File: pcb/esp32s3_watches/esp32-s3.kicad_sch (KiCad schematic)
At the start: 14 parts, among them J2 10067847-001RLF, U1 ESP32-S3-DevKitC, U4 SW_DPDT_XLX

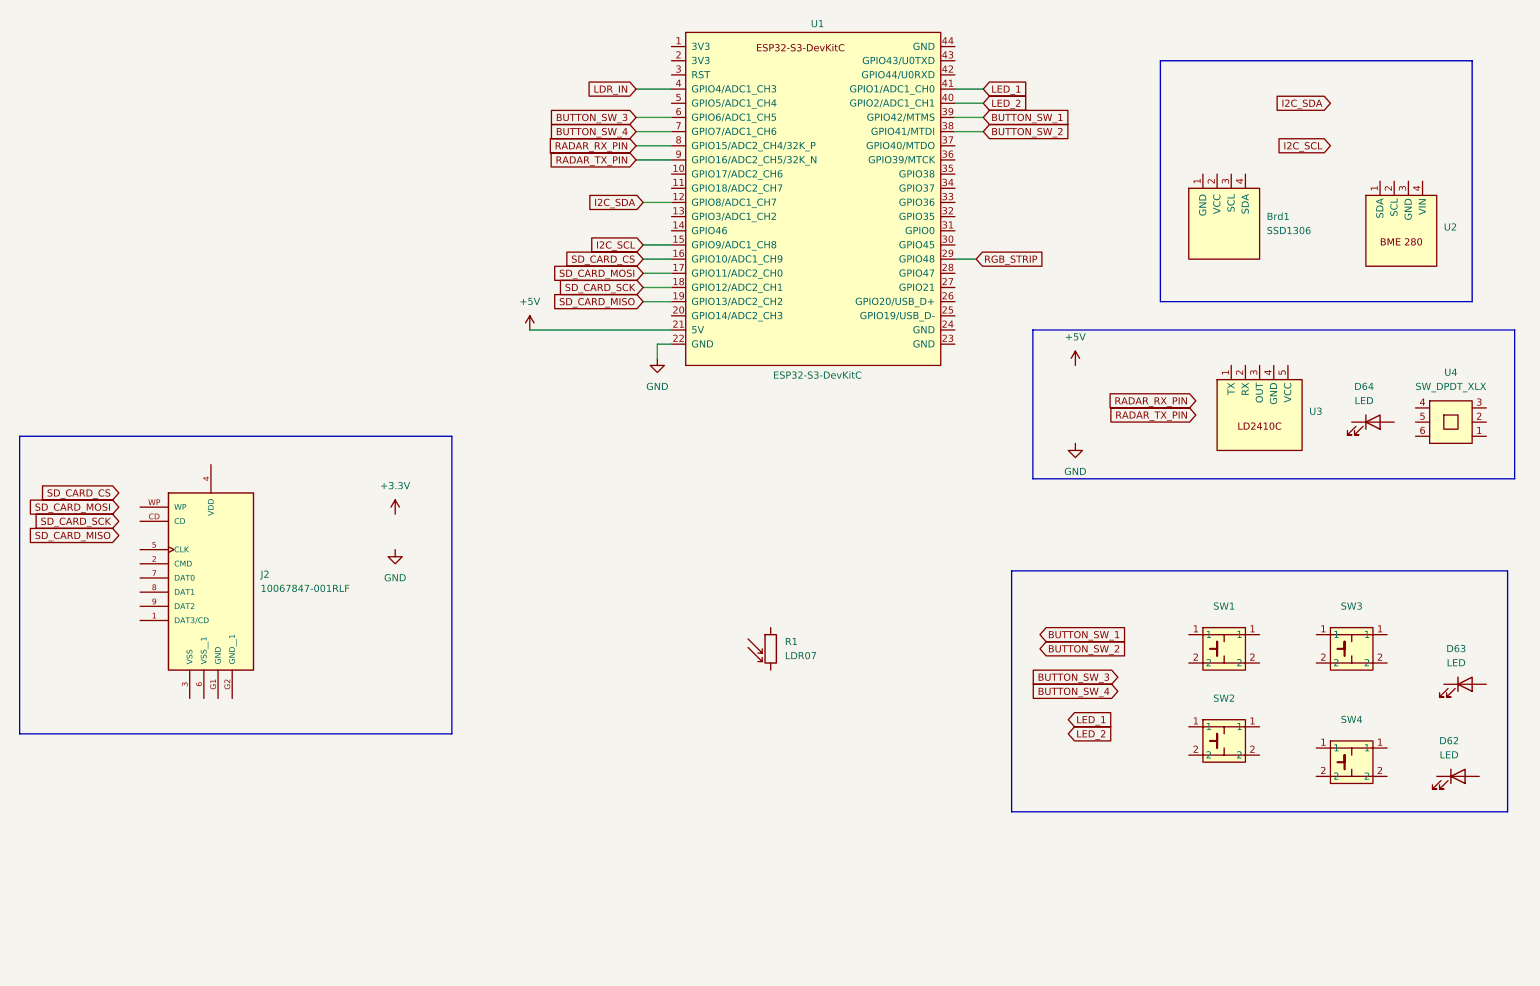
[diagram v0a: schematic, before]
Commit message: Scheme improvements
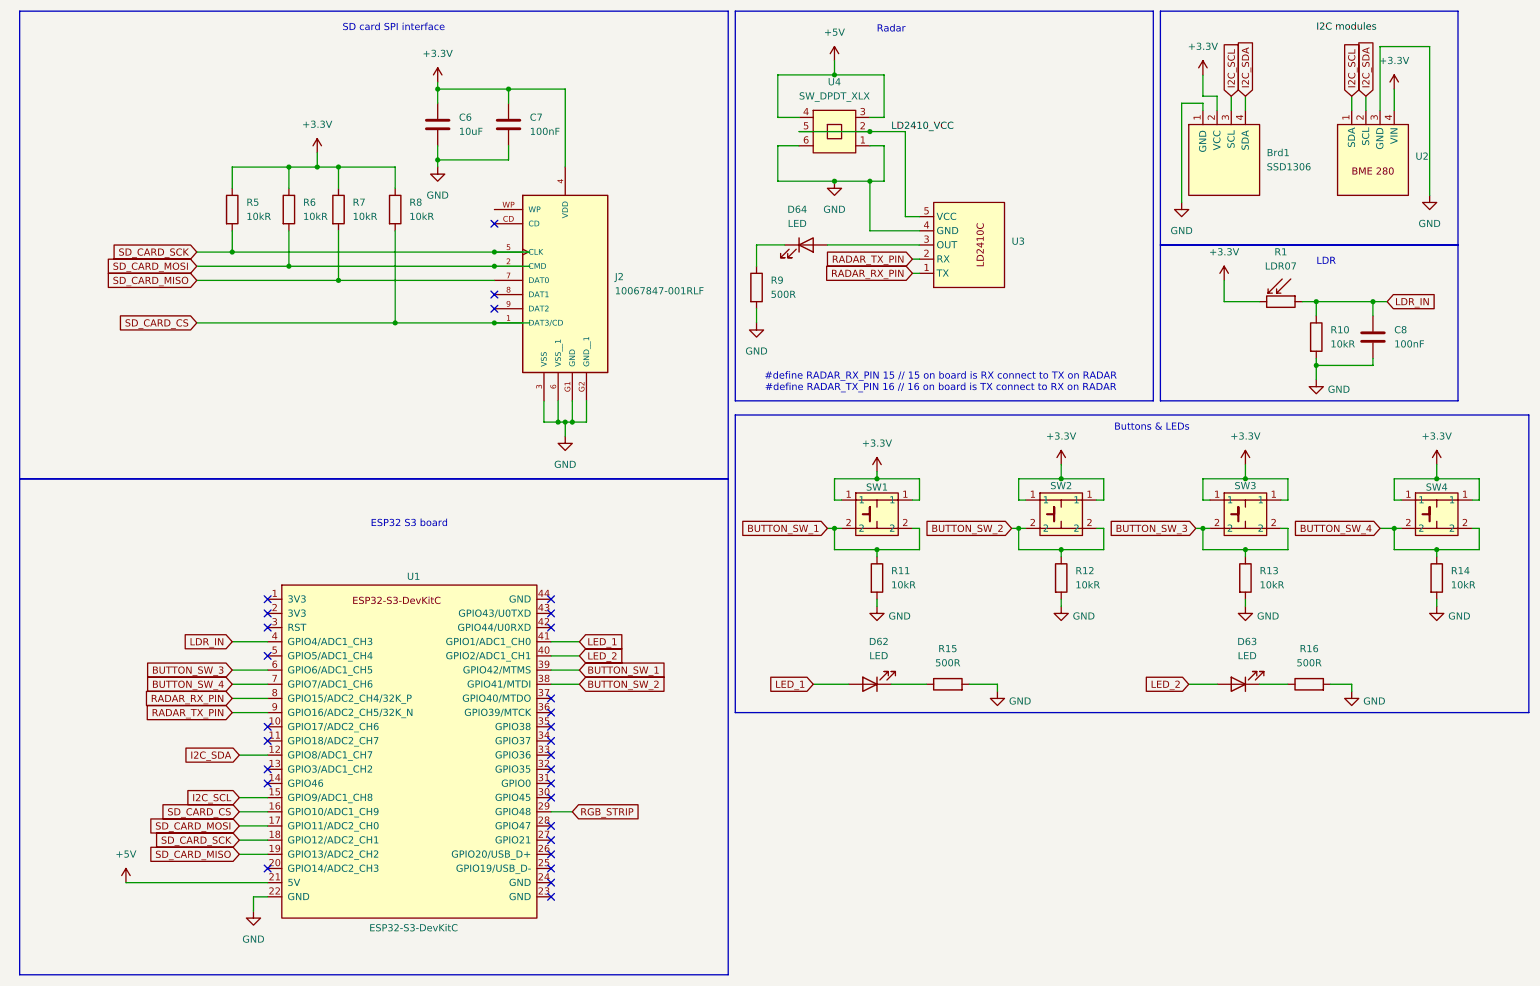
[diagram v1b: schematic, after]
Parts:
- added C6: 10uF, symbol Device:C
- added C7, C8: 100nF, symbol Device:C
- added R10, R11, R12, R13, R14, R5, R6, R7, R8: 10kR, symbol Device:R
- added R15, R16, R9: 500R, symbol Device:R
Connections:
- net +3.3V: now also Brd1.2 (VCC), J2.4 (VDD), R1.2, SW1.1, SW2.1, SW3.1, SW4.1, U2.4 (VIN), C6.1, C7.1, R5.1, R6.1, R7.1, R8.1
- net +5V: now also U4.3, U4.4
- net BUTTON_SW_1: now also SW1.2, R11.1
- net BUTTON_SW_2: now also SW2.2, R12.1
- net BUTTON_SW_3: now also SW3.2, R13.1
- net BUTTON_SW_4: now also SW4.2, R14.1
- net GND: now also Brd1.1 (GND), J2.3 (VSS), J2.6 (VSS__1), J2.G1 (GND), J2.G2 (GND__1), U2.3 (GND), U3.4 (GND), U4.1, U4.6, C6.2, C7.2, C8.2, R10.2, R11.2, R12.2, R13.2, R14.2, R15.2, R16.2, R9.2
- net I2C_SCL: now also Brd1.3 (SCL), U2.1 (SDA)
- net I2C_SDA: now also Brd1.4 (SDA), U2.2 (SCL)
- net LDR_IN: now also R1.1, C8.1, R10.1
- net LED_1: now also D62.2 (A)
- net LED_2: now also D63.2 (A)
- net RADAR_RX_PIN: now also U3.1 (TX)
- net RADAR_TX_PIN: now also U3.2 (RX)
- net SD_CARD_CS: now also J2.1 (DAT3/CD), R8.2
- net SD_CARD_MISO: now also J2.7 (DAT0), R7.2
- net SD_CARD_MOSI: now also J2.2 (CMD), R6.2
- net SD_CARD_SCK: now also J2.5 (CLK), R5.2
- net at D62.1 (K): now also R15.1
- net at D63.1 (K): now also R16.1
- net at D64.1 (K): now also R9.1
- net at D64.2 (A): now also U3.3 (OUT)
- net LD2410_VCC: now reaches U4.2
- net LD2410_VCC: now also U3.5 (VCC), U4.5
- no-connect marks 0 -> 29
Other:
- note added: "#define RADAR_RX_PIN 15 // 15 on board is RX connect to TX on RADAR #define RADAR_TX_PIN 16 // 16 on board is TX connect to RX on RADAR"
- note added: "Buttons & LEDs"
- note added: "ESP32 S3 board"
- note added: "LDR"
- note added: "Radar"
- note added: "SD card SPI interface"
- moved on the sheet: Brd1, D62, D63, D64, J2, R1, SW1, SW2, SW3, SW4, U1, U2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
